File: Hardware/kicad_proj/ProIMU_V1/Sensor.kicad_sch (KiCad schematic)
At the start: 9 parts, among them U5 MPU-9250, U6 BMP280

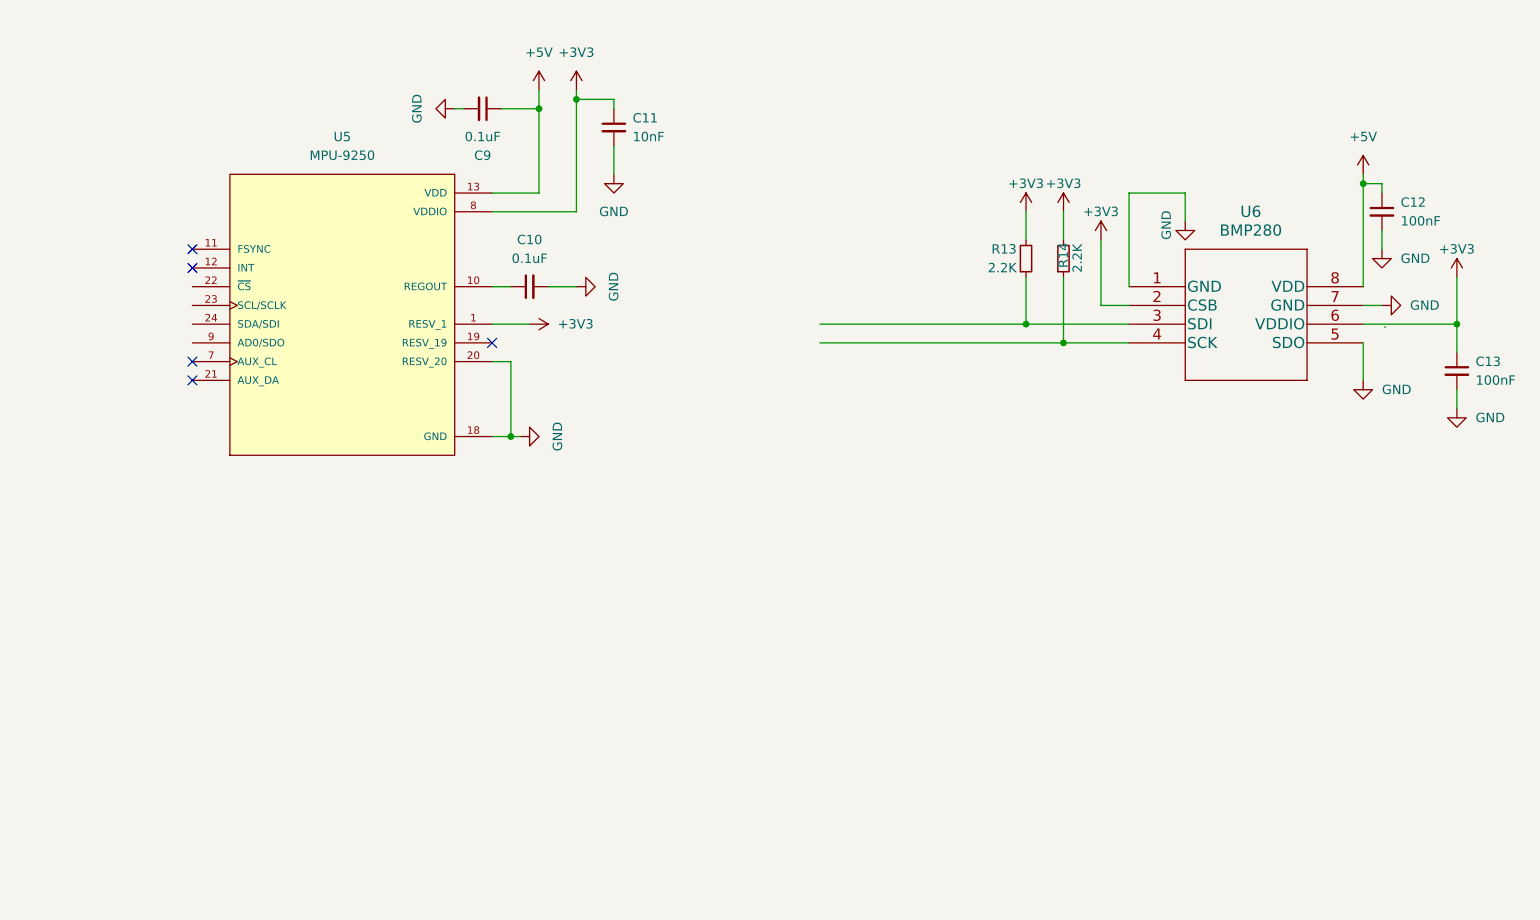
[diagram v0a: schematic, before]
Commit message: Updated Repo
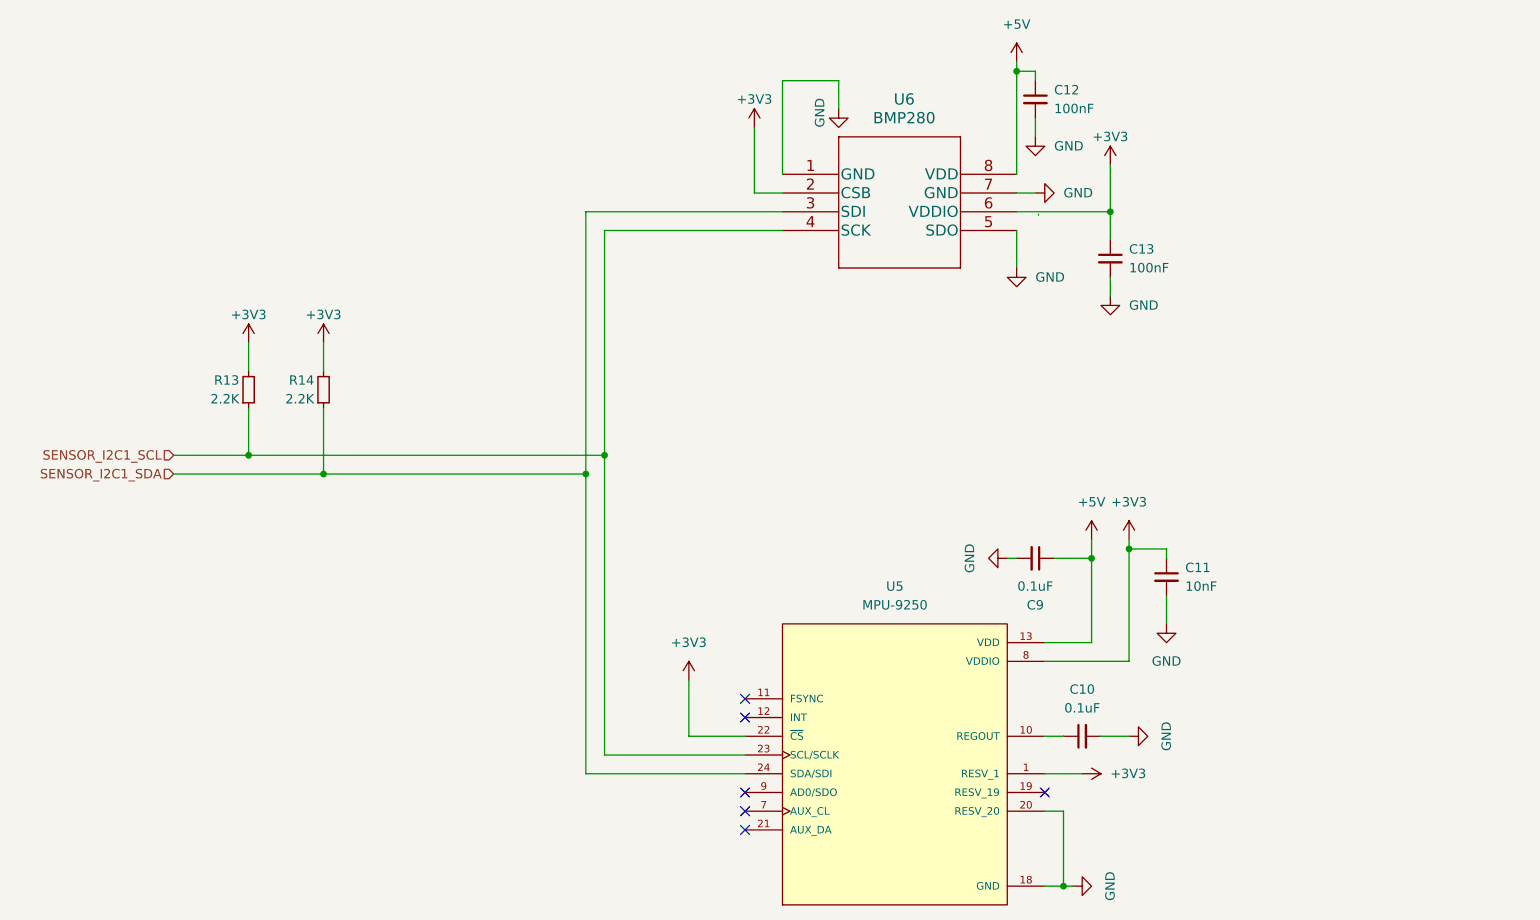
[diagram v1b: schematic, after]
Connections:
- net +3V3: now also U5.22 (~{CS})
- net SENSOR_I2C1_SCL: now reaches U6.4 (SCK)
- net SENSOR_I2C1_SCL: now also R13.1, U5.23 (SCL/SCLK); no longer R14.1
- net SENSOR_I2C1_SDA: now reaches U5.24 (SDA/SDI)
- net SENSOR_I2C1_SDA: now also R14.1, U6.3 (SDI)
- no-connect marks 5 -> 6
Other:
- moved on the sheet: C10, C11, C12, C13, C9, R13, U5, U6
